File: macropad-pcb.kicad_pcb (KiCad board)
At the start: 2 copper layers, 75 x 35 mm, 12 parts

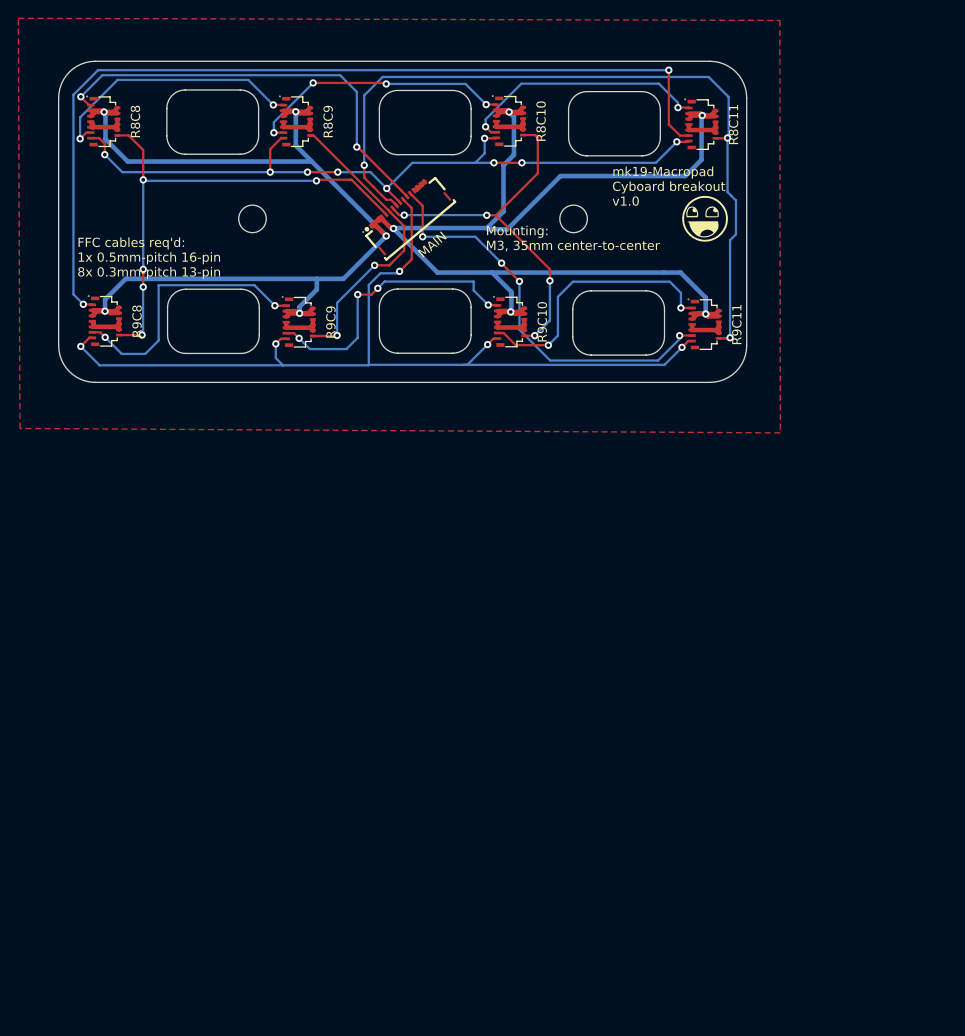
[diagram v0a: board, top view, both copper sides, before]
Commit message: rev2 ready for sleeping on
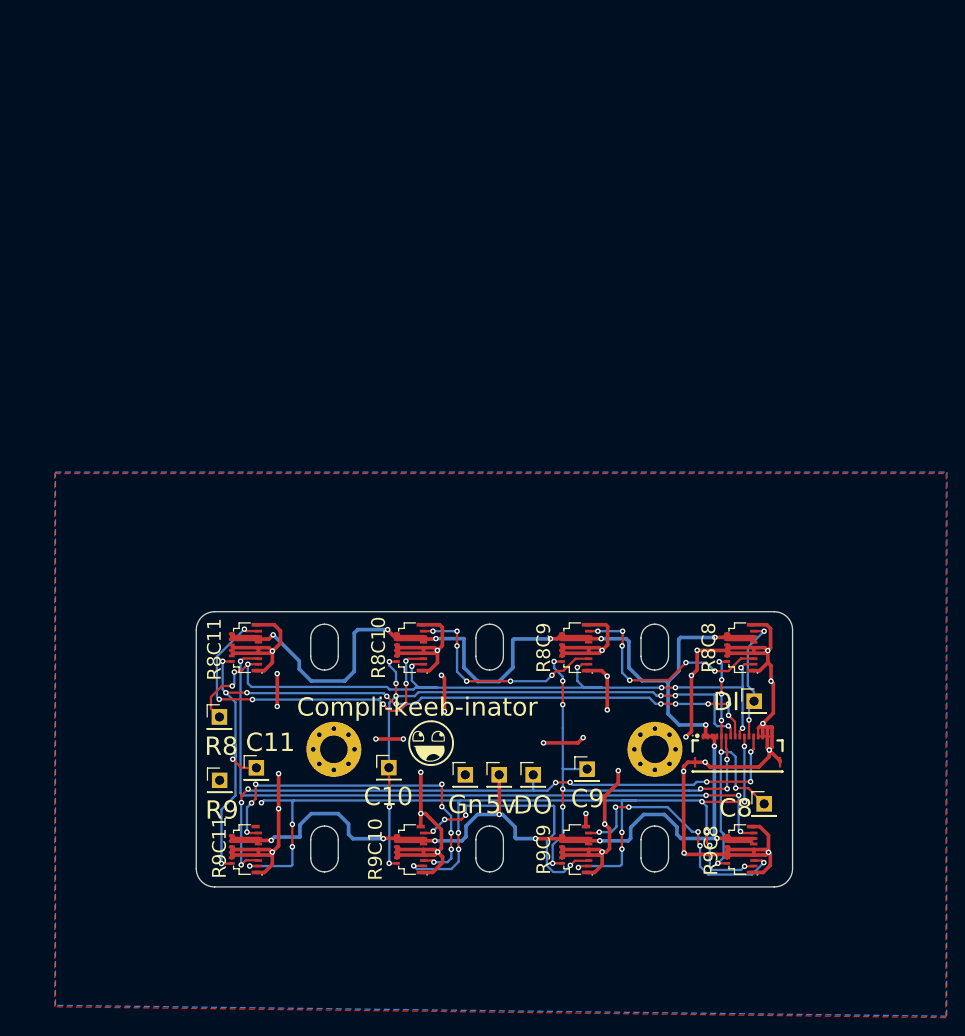
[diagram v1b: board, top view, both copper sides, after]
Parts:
- removed G***: LOGO, ct-kicad:awesome-logo
- removed MAIN: HC-FPC-05-10-16RLTAG, ct-kicad:FPC-SMD_16P-P0.50_HCTL_HC-FPC-05-10-16RLTAG
- added J1: Conn_01x01_Socket, Connector_PinHeader_2.54mm:PinHeader_1x01_P2.54mm_Vertical, F.Cu at (176.9, 106.0)
- added J10: Conn_01x01_Socket, Connector_PinHeader_2.54mm:PinHeader_1x01_P2.54mm_Vertical, F.Cu at (144.3, 102.8)
- added J2: Conn_01x01_Socket, Connector_PinHeader_2.54mm:PinHeader_1x01_P2.54mm_Vertical, F.Cu at (157.6, 102.2)
- added J3: Conn_01x01_Socket, Connector_PinHeader_2.54mm:PinHeader_1x01_P2.54mm_Vertical, F.Cu at (136.0, 102.0)
- added J4: Conn_01x01_Socket, Connector_PinHeader_2.54mm:PinHeader_1x01_P2.54mm_Vertical, F.Cu at (121.5, 102.0)
- added J5: Conn_01x01_Socket, Connector_PinHeader_2.54mm:PinHeader_1x01_P2.54mm_Vertical, F.Cu at (151.7, 102.8)
- added J6: Conn_01x01_Socket, Connector_PinHeader_2.54mm:PinHeader_1x01_P2.54mm_Vertical, F.Cu at (117.5, 96.5)
- added J7: Conn_01x01_Socket, Connector_PinHeader_2.54mm:PinHeader_1x01_P2.54mm_Vertical, F.Cu at (117.5, 103.4)
- added J8: Conn_01x01_Socket, Connector_PinHeader_2.54mm:PinHeader_1x01_P2.54mm_Vertical, F.Cu at (175.8, 94.8)
- added J9: Conn_01x01_Socket, Connector_PinHeader_2.54mm:PinHeader_1x01_P2.54mm_Vertical, F.Cu at (148.0, 102.8)
- added LOGO1: **REF, ct-kicad:awesome-logo, F.Cu at (140.6, 99.3)
- added LOGO2: **REF, ct-kicad:qmk-lite, B.Cu at (147.8, 100.0)
- added MAIN1: HC-FPC-05-10-16RLTAG, ct-kicad:FPC-SMD_16P-P0.50_HCTL_HC-FPC-05-10-16RLTAG, F.Cu at (174.0, 100.0)
- H1, H2: footprint MountingHole:MountingHole_3mm -> MountingHole:MountingHole_3mm_Pad_Via
- moved R9C8 90.0 mm to (174.3, 110.9), turned to 90 degrees
- moved R8C8 90.0 mm to (174.3, 88.9), turned to 90 degrees
- moved R9C11 76.1 mm to (120.3, 110.9), turned to 90 degrees
- moved R8C11 75.7 mm to (120.3, 88.9), turned to 90 degrees
- moved R8C9 64.9 mm to (156.3, 88.9), turned to 90 degrees
- moved R9C9 64.9 mm to (156.3, 110.9), turned to 90 degrees
- moved R9C10 58.5 mm to (138.3, 110.9), turned to 90 degrees
- moved H1 58.5 mm to (130.0, 100.0)
- moved H2 58.5 mm to (165.0, 100.0)
- moved R8C10 58.4 mm to (138.3, 88.9), turned to 90 degrees
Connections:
- R8C10 pad 1: Net-(P3-Pad11) -> row8
- R8C10 pad 10: GND -> VCC
- R8C10 pad 11: Net-(P5-Pad11) -> VCC
- R8C10 pad 12: col10 -> VCC
- R8C10 pad 13: row8 -> Net-(R8C10-Pad13)
- R8C10 pad 14: unconnected-(P5-Pad14) -> GND
- R8C10 pad 15: unconnected-(P5-Pad15) -> GND
- R8C10 pad 2: VCC -> col10
- R8C10 pad 3: VCC -> Net-(R8C10-Pad3)
- R8C10 pad 4: VCC -> GND
- R8C10 pad 5: VCC -> GND
- R8C10 pad 9: GND -> VCC
- R8C11 pad 1: Net-(P5-Pad11) -> row8
- R8C11 pad 10: GND -> VCC
- R8C11 pad 11: from_row_9_DO -> VCC
- R8C11 pad 12: col11 -> VCC
- R8C11 pad 13: row8 -> Net-(R8C10-Pad3)
- R8C11 pad 14: unconnected-(P7-Pad14) -> GND
- R8C11 pad 15: unconnected-(P7-Pad15) -> GND
- R8C11 pad 2: VCC -> col11
- R8C11 pad 3: VCC -> from_row_9_DO
- R8C11 pad 4: VCC -> GND
- R8C11 pad 5: VCC -> GND
- R8C11 pad 9: GND -> VCC
- R8C8 pad 1: Net-(P1-Pad1) -> row8
- R8C8 pad 10: GND -> VCC
- R8C8 pad 11: Net-(P1-Pad11) -> VCC
- R8C8 pad 12: col8 -> VCC
- R8C8 pad 13: row8 -> LED_DI
- R8C8 pad 14: unconnected-(P1-Pad14) -> GND
- R8C8 pad 15: unconnected-(P1-Pad15) -> GND
- R8C8 pad 2: VCC -> col8
- R8C8 pad 3: VCC -> Net-(R8C8-Pad3)
- R8C8 pad 4: VCC -> GND
- R8C8 pad 5: VCC -> GND
- R8C8 pad 9: GND -> VCC
- R8C9 pad 1: Net-(P1-Pad11) -> row8
- R8C9 pad 10: GND -> VCC
- R8C9 pad 11: Net-(P3-Pad11) -> VCC
- R8C9 pad 12: col9 -> VCC
- R8C9 pad 13: row8 -> Net-(R8C8-Pad3)
- R8C9 pad 14: unconnected-(P3-Pad14) -> GND
- R8C9 pad 15: unconnected-(P3-Pad15) -> GND
- R8C9 pad 2: VCC -> col9
- R8C9 pad 3: VCC -> Net-(R8C10-Pad13)
- R8C9 pad 4: VCC -> GND
- R8C9 pad 5: VCC -> GND
- R8C9 pad 9: GND -> VCC
- R9C10 pad 1: Net-(P4-Pad11) -> row9
- R9C10 pad 10: GND -> VCC
- R9C10 pad 11: Net-(P6-Pad11) -> VCC
- R9C10 pad 12: col10 -> VCC
- R9C10 pad 13: row9 -> Net-(R9C10-Pad13)
- R9C10 pad 14: unconnected-(P6-Pad14) -> GND
- R9C10 pad 15: unconnected-(P6-Pad15) -> GND
- R9C10 pad 2: VCC -> col10
- R9C10 pad 3: VCC -> Net-(R9C10-Pad3)
- R9C10 pad 4: VCC -> GND
- R9C10 pad 5: VCC -> GND
- R9C10 pad 9: GND -> VCC
- R9C11 pad 1: Net-(P6-Pad11) -> row9
- R9C11 pad 10: GND -> VCC
- R9C11 pad 11: LED_DO_MACRO -> VCC
- R9C11 pad 12: col11 -> VCC
- R9C11 pad 13: row9 -> Net-(R9C10-Pad3)
- R9C11 pad 14: unconnected-(P8-Pad14) -> GND
- R9C11 pad 15: unconnected-(P8-Pad15) -> GND
- R9C11 pad 2: VCC -> col11
- R9C11 pad 3: VCC -> LED_DO_MACRO
- R9C11 pad 4: VCC -> GND
- R9C11 pad 5: VCC -> GND
- R9C11 pad 9: GND -> VCC
- R9C8 pad 1: from_row_9_DO -> row9
- R9C8 pad 10: GND -> VCC
- R9C8 pad 11: Net-(P2-Pad11) -> VCC
- R9C8 pad 12: col8 -> VCC
- R9C8 pad 13: row9 -> from_row_9_DO
- R9C8 pad 14: unconnected-(P2-Pad14) -> GND
- R9C8 pad 15: unconnected-(P2-Pad15) -> GND
- R9C8 pad 2: VCC -> col8
- R9C8 pad 3: VCC -> Net-(R9C8-Pad3)
- R9C8 pad 4: VCC -> GND
- R9C8 pad 5: VCC -> GND
- R9C8 pad 9: GND -> VCC
- R9C9 pad 1: Net-(P2-Pad11) -> row9
- R9C9 pad 10: GND -> VCC
- R9C9 pad 11: Net-(P4-Pad11) -> VCC
- R9C9 pad 12: col9 -> VCC
- R9C9 pad 13: row9 -> Net-(R9C8-Pad3)
- R9C9 pad 14: unconnected-(P4-Pad14) -> GND
- R9C9 pad 15: unconnected-(P4-Pad15) -> GND
- R9C9 pad 2: VCC -> col9
- R9C9 pad 3: VCC -> Net-(R9C10-Pad13)
- R9C9 pad 4: VCC -> GND
- R9C9 pad 5: VCC -> GND
- R9C9 pad 9: GND -> VCC
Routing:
- net GND: track 38.7 -> 251.9 mm, vias 0 -> 34
- net Net-(P1-Pad1): track 47.0 -> 0.00 mm, vias 2 -> 0
- net Net-(R9C10-Pad3): track 0.00 -> 39.1 mm, vias 0 -> 8
- net Net-(R8C10-Pad3): track 0.00 -> 38.6 mm, vias 0 -> 6
- net Net-(P4-Pad11): track 31.2 -> 0.00 mm, vias 4 -> 0
- net Net-(P2-Pad11): track 29.7 -> 0.00 mm, vias 2 -> 0
- net VCC: track 238.4 -> 209.0 mm, vias 10 -> 15
- net Net-(P6-Pad11): track 29.3 -> 0.00 mm, vias 2 -> 0
- net Net-(P3-Pad11): track 29.2 -> 0.00 mm, vias 4 -> 0
- net Net-(P1-Pad11): track 28.8 -> 0.00 mm, vias 2 -> 0
- net Net-(R9C8-Pad3): track 0.00 -> 28.5 mm, vias 0 -> 6
- net LED_DO_MACRO: track 44.7 -> 73.0 mm, vias 4 -> 8
- net Net-(R9C10-Pad13): track 0.00 -> 28.3 mm, vias 0 -> 4
- net Net-(P5-Pad11): track 27.4 -> 0.00 mm, vias 2 -> 0
- net Net-(R8C8-Pad3): track 0.00 -> 24.7 mm, vias 0 -> 6
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- added copper zone on B.Cu, net GND
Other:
- board size 75 x 35 mm -> 65 x 30 mm
- board text added: "5v"
- board text added: "C10"
- board text added: "C11"
- board text added: "C8"
- board text added: "C9"
- board text added: "Compli-keeb-inator"
- board text added: "DI"
- board text added: "DO"
- board text added: "Gn"
- board text added: "R8"
- board text added: "R9"
- board text removed: "FFC cables req'd: 1x 0.5mm-pitch 16-pin 8x 0.3mm-pitch 13-pin"
- board text removed: "Mounting: M3, 35mm center-to-center"
- board text removed: "mk19-Macropad Cyboard breakout v1.0"
